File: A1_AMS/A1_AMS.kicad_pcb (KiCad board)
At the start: 2 copper layers, 60 x 60 mm, 19 parts, among them J1 Screw_Terminal_01x02, J2 Servo, J3 9-10-11-14-15, J4 Conn_01x04, J5 16-17-18-19-20, J6 21-22-26-27-28, J7 Conn_01x04, J8 5-5-3.3-G-G, M1 StepperMotor, M2 StepperMotor, U1 Pico

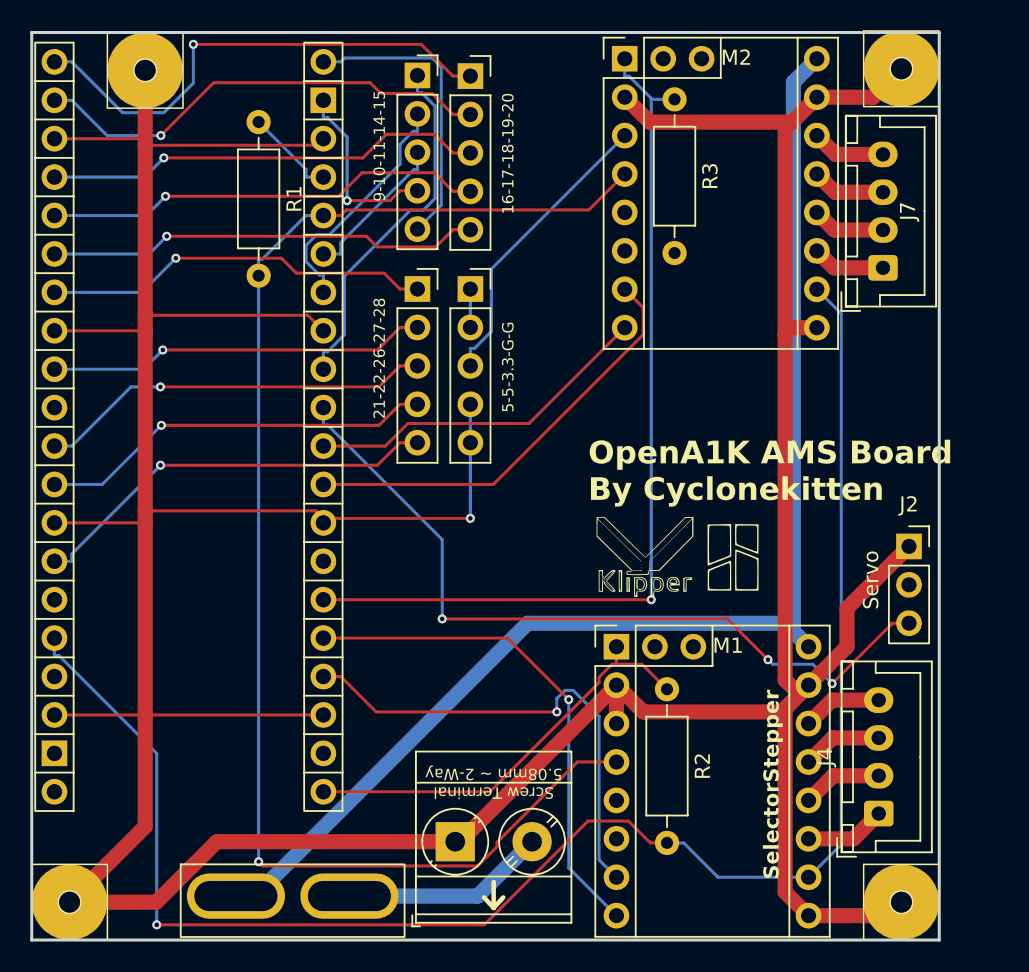
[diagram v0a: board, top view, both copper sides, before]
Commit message: e
e
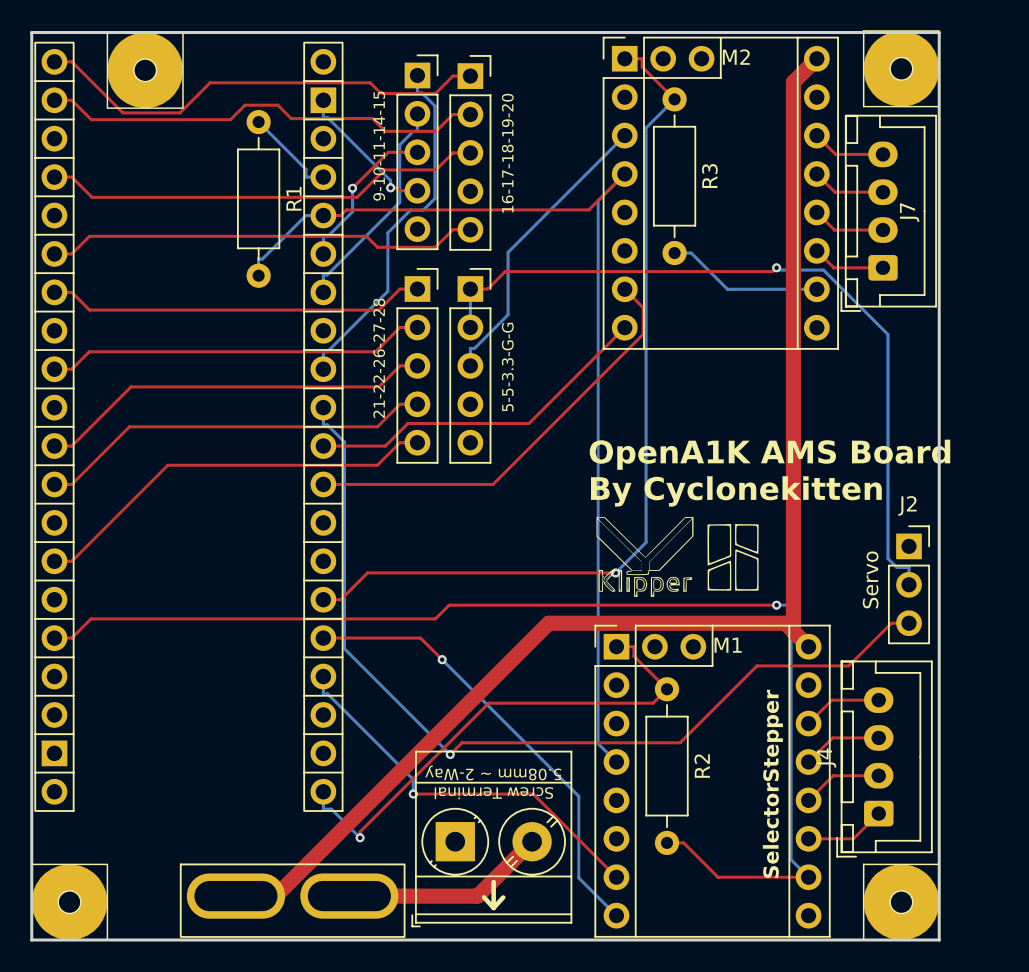
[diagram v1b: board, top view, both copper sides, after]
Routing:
- net GND: track 303.8 -> 0.00 mm, vias 1 -> 0
- net /5V: track 2.54 -> 50.2 mm, vias 0 -> 1
- net /G19: track 29.2 -> 0.00 mm, vias 1 -> 0
- net /M_UART: track 93.2 -> 67.7 mm, vias 1 -> 0
- net /G15: track 19.5 -> 0.00 mm
- net /SV_SIG: track 51.7 -> 60.5 mm, vias 3 -> 1
- net /MS_STEP: track 32.1 -> 26.1 mm
- net /MS_EN: track 28.3 -> 33.8 mm, vias 0 -> 1
- net /MS_DIR: track 33.5 -> 30.1 mm
- net /G14: track 12.4 -> 9.65 mm
- net /G16: track 33.1 -> 30.5 mm, vias 1 -> 0
- net /MD_EN: track 59.9 -> 57.7 mm
- net /G10: track 16.1 -> 14.7 mm
- net /G17: track 30.8 -> 29.6 mm, vias 1 -> 0
- net /G21: track 25.8 -> 25.1 mm, vias 1 -> 0
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- added copper zone on B.Cu, net GND
- added copper zone on F.Cu, net GND
